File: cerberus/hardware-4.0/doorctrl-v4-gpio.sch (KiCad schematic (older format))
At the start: 20 parts, among them CON3 RJHSE-5085, CON4 RJHSE-5085, CON5 RJHSE-5085, K1 G5SB, P1 CONN_2_V

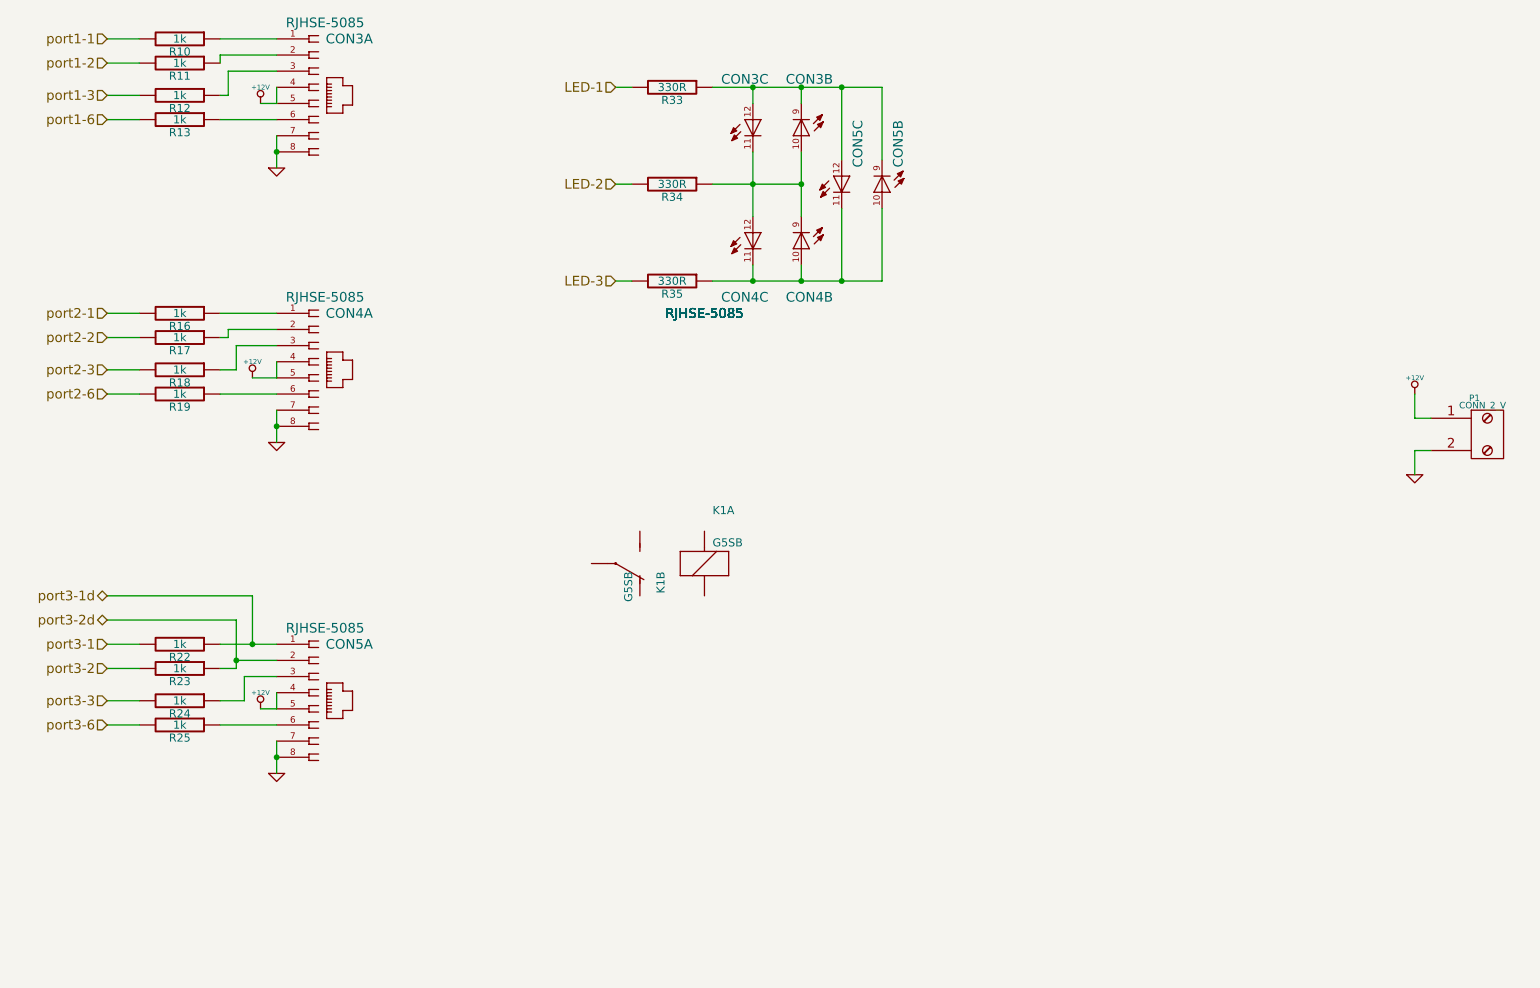
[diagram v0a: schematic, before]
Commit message: Blaarghle
git-svn-id: file:///home/ff/projects/osaa/svn@212 a092026d-3e22-4cff-94a7-eaa6fdd35d37
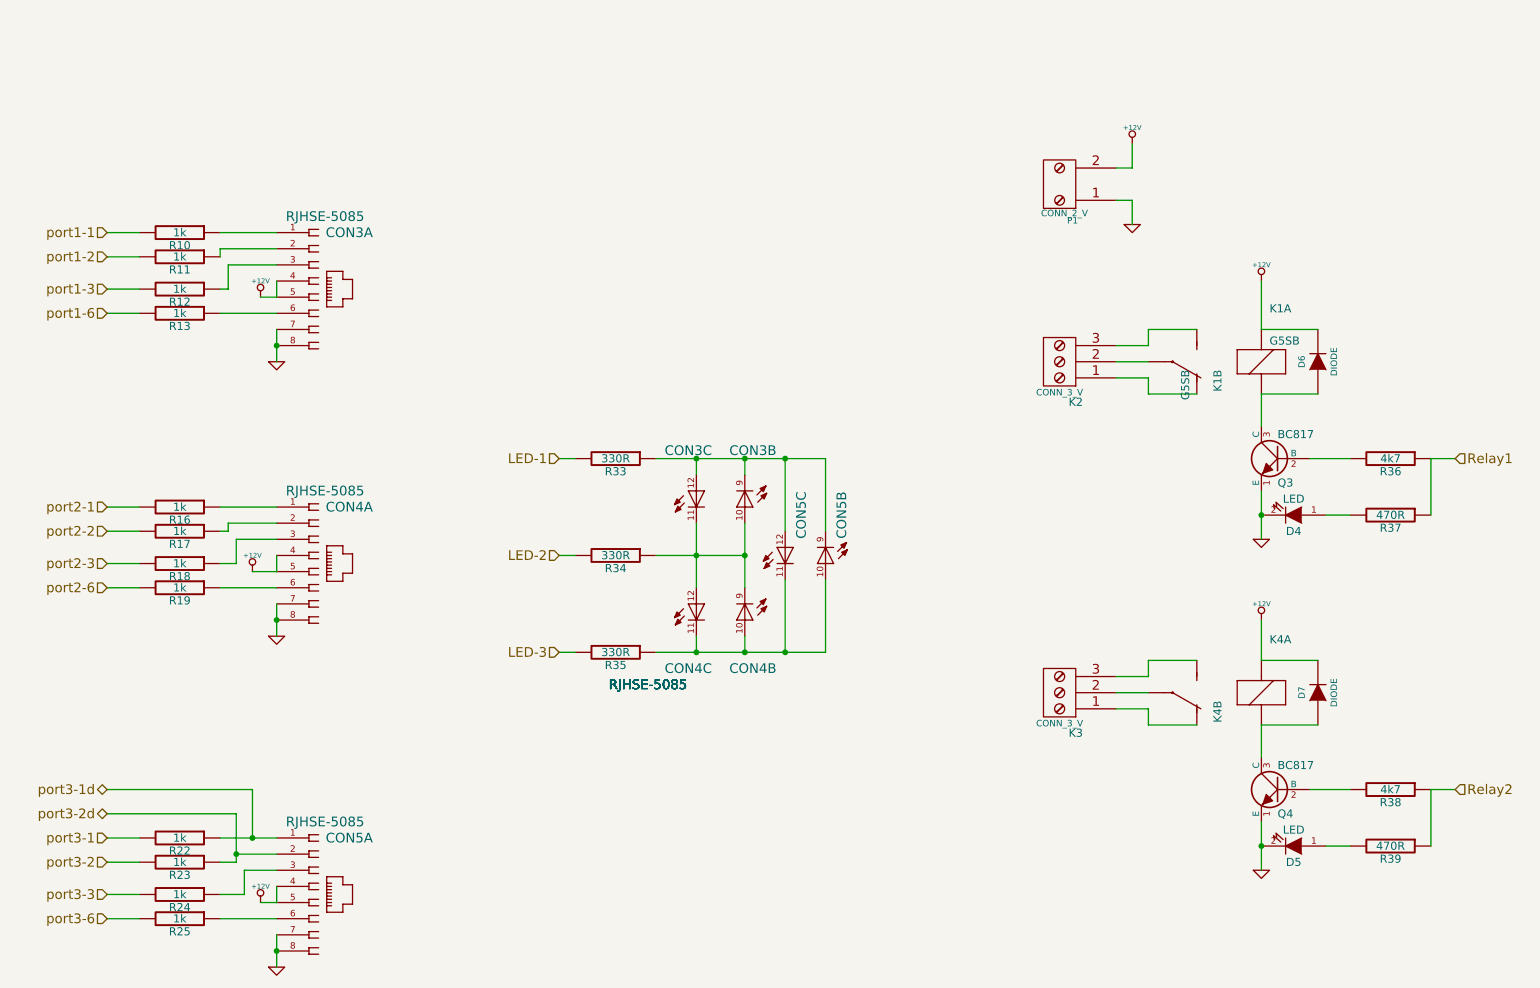
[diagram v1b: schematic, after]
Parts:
- added D4, D5: LED, symbol LED
- added D6, D7: DIODE, symbol DIODE
- added K2, K3: CONN_3_V, symbol CONN_3_V
- added K4: G5SB, g5sb, symbol G5SB
- added Q3, Q4: BC817, symbol NPN
- added R36, R38: 4k7, symbol R
- added R37, R39: 470R, symbol R
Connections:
- net +12V: now also K1.1, P1.2 (P2), D6.2 (K), D7.2 (K), K4.1; no longer P1.1 (P1)
- net GND: now also P1.1 (P1), D4.2 (K), D5.2 (K), Q3.1 (E), Q4.1 (E); no longer P1.2 (P2)
- net at K1.5 (2): now also D6.1 (A), Q3.3 (C)
- net at K1.2 (P): now also K2.2 (P2)
- net at K1.3 (S): now also K2.3 (P3)
- net at K1.4 (O): now also K2.1 (P1)
- new net: Q3.2 (B), R36.2
- new net: D4.1 (A), R37.2
- new net: D7.1 (A), K4.5 (2), Q4.3 (C)
- new net: K3.2 (P2), K4.2 (P)
- new net: K3.3 (P3), K4.3 (S)
- new net: K3.1 (P1), K4.4 (O)
- new net: Q4.2 (B), R38.2
- new net: D5.1 (A), R39.2
- new net Relay1: R36.1, R37.1
- new net Relay2: R38.1, R39.1
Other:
- moved on the sheet: CON3A, CON3B, CON3C, CON4A, CON4B, CON4C, CON5A, CON5B, CON5C, K1A, K1B, P1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
